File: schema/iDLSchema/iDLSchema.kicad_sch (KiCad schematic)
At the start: 11 parts, among them U1 HC-SR04, U2 HC-SR04, U3 HC-SR04

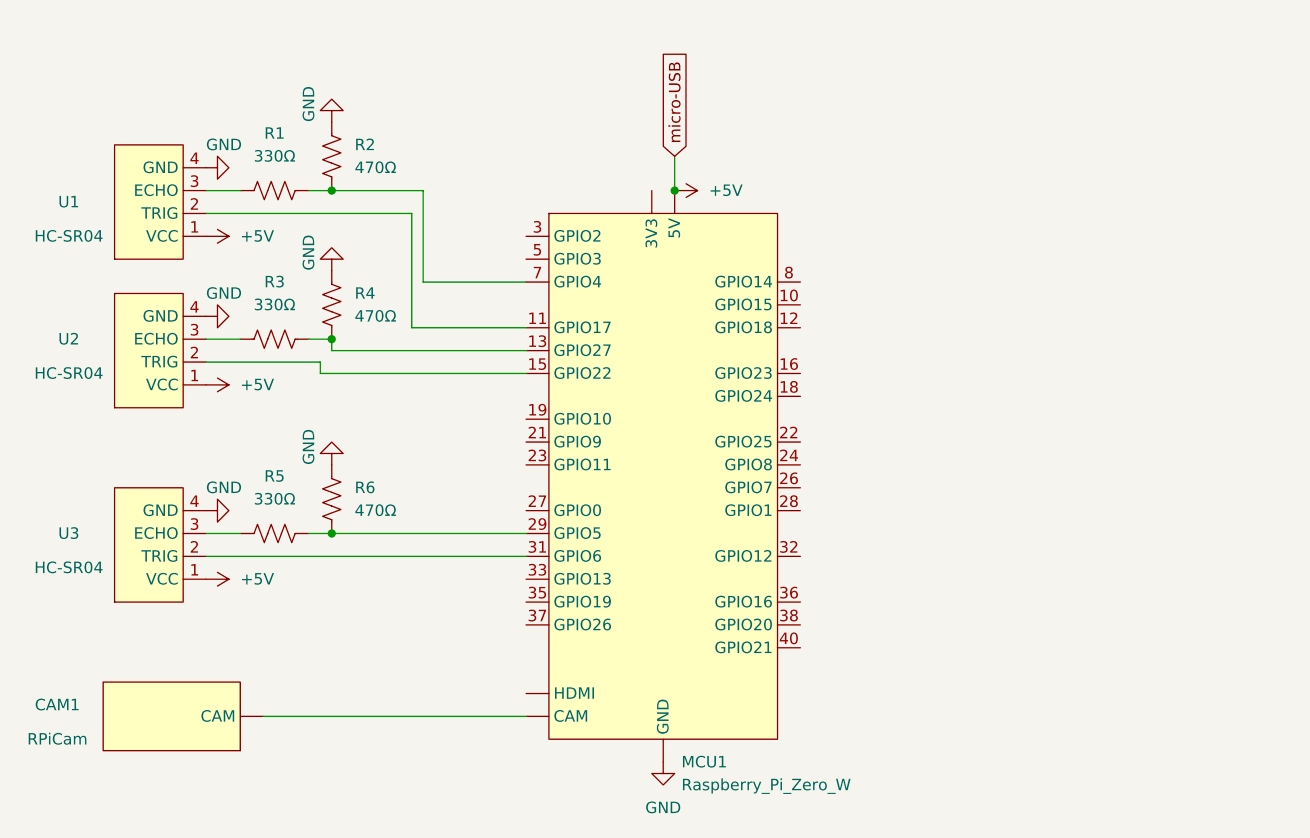
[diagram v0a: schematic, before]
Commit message: schema v0.2
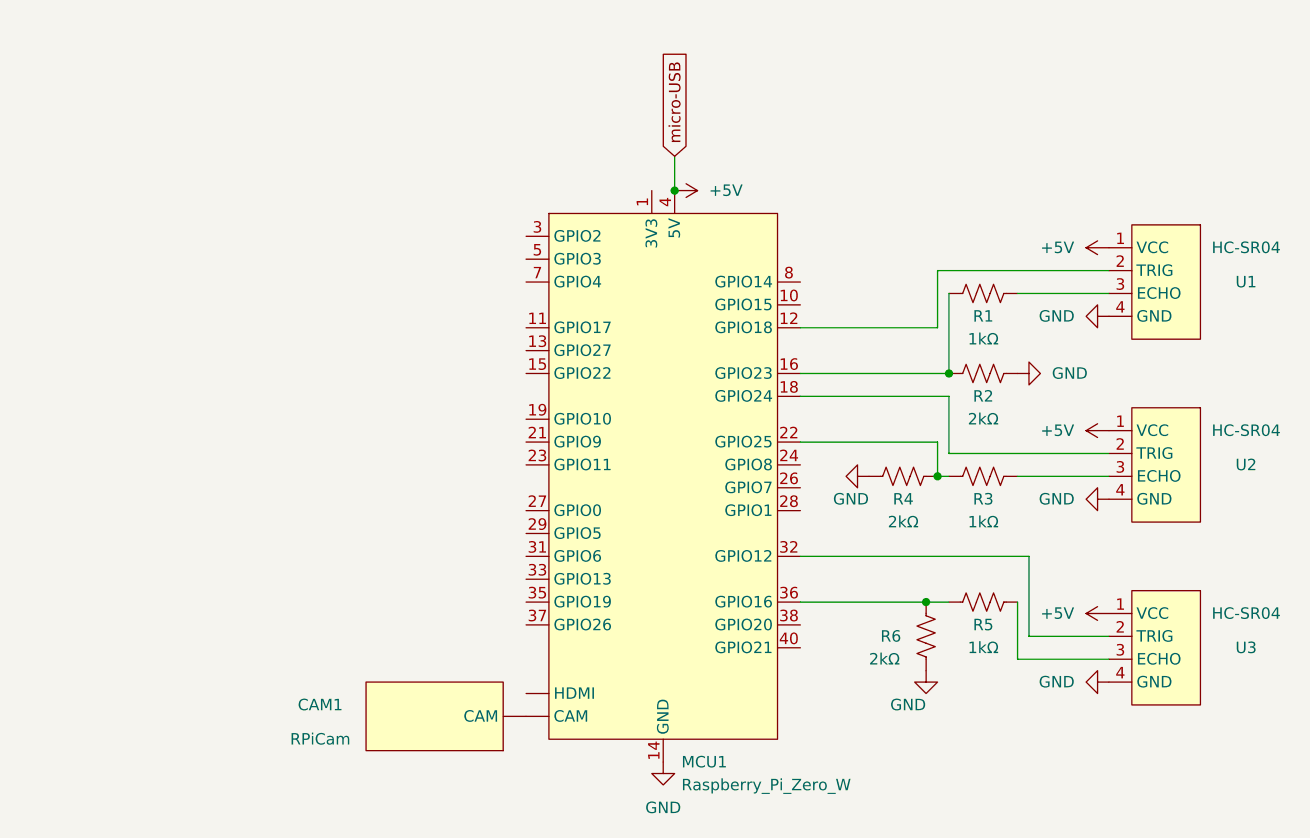
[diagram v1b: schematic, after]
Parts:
- R1, R3, R5: value 330Ω -> 1kΩ
- R2, R4, R6: value 470Ω -> 2kΩ
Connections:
- net +5V: now also MCU1.4 (5V); no longer MCU1. (HDMI)
- net GND: now also MCU1.14 (GND), R2.1, R4.2; no longer MCU1. (HDMI), R2.2, R4.1
- net at MCU1. (HDMI): now also CAM1. (CAM)
- net at MCU1.11 (GPIO17): no longer U1.2 (TRIG)
- net at MCU1.12 (GPIO18): now also U1.2 (TRIG)
- net at MCU1.15 (GPIO22): no longer U2.2 (TRIG)
- net at MCU1.16 (GPIO23): now also R1.2, R2.2
- net at MCU1.18 (GPIO24): now also U2.2 (TRIG)
- net at MCU1.22 (GPIO25): now also R3.2, R4.1
- net at R5.2, R6.1: now also MCU1.36 (GPIO16); no longer MCU1.29 (GPIO5)
- net at MCU1.31 (GPIO6): no longer U3.2 (TRIG)
- net at MCU1.32 (GPIO12): now also U3.2 (TRIG)
- net at U2.3 (ECHO): now also R3.1; no longer R3.2
- now unconnected: MCU1.13 (GPIO27), MCU1.7 (GPIO4)
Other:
- moved on the sheet: CAM1, U1, U3
